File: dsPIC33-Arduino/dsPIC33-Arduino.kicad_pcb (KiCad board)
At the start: 2 copper layers, 68.6 x 53.3 mm, 58 parts, among them CON1 BARREL_JACK, P1 Power, P10 PIN20, P11 PIN5, P12 PWR_IN, P13 PIN2, P14 Power Select, P15 I2C, P16 PIN19, P17 UART/CAN, P2 Analog, P3 Digital, P4 Digital, P5 CONN_1, P6 CONN_1, P7 CONN_1, P8 CONN_1, P9 USB_B, SW1 SW_PUSH, U1 FT230XS, U2 LM1117 3V3, U3 dsPIC33EVxxxGM102-I/SP, U4 74LVC1G32, U5 LM1117 5V, Y1 Crystal

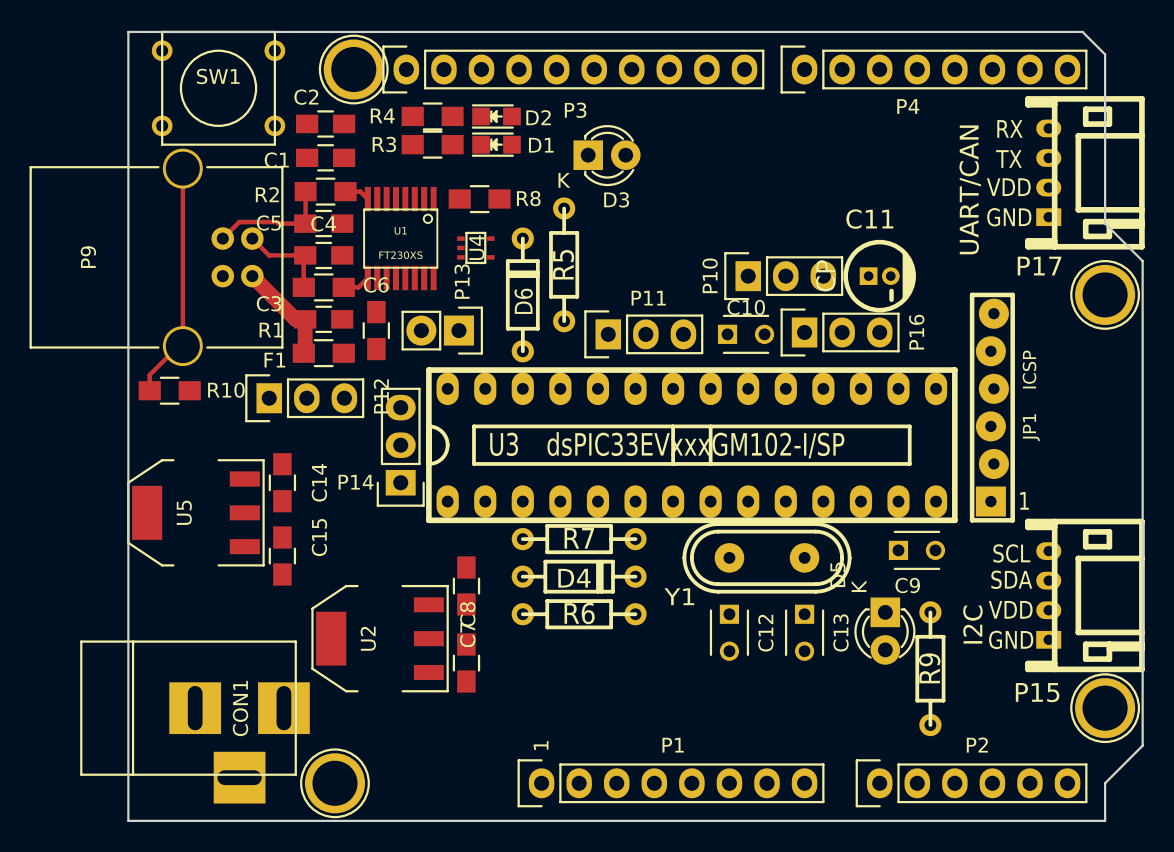
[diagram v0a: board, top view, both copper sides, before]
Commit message: wip
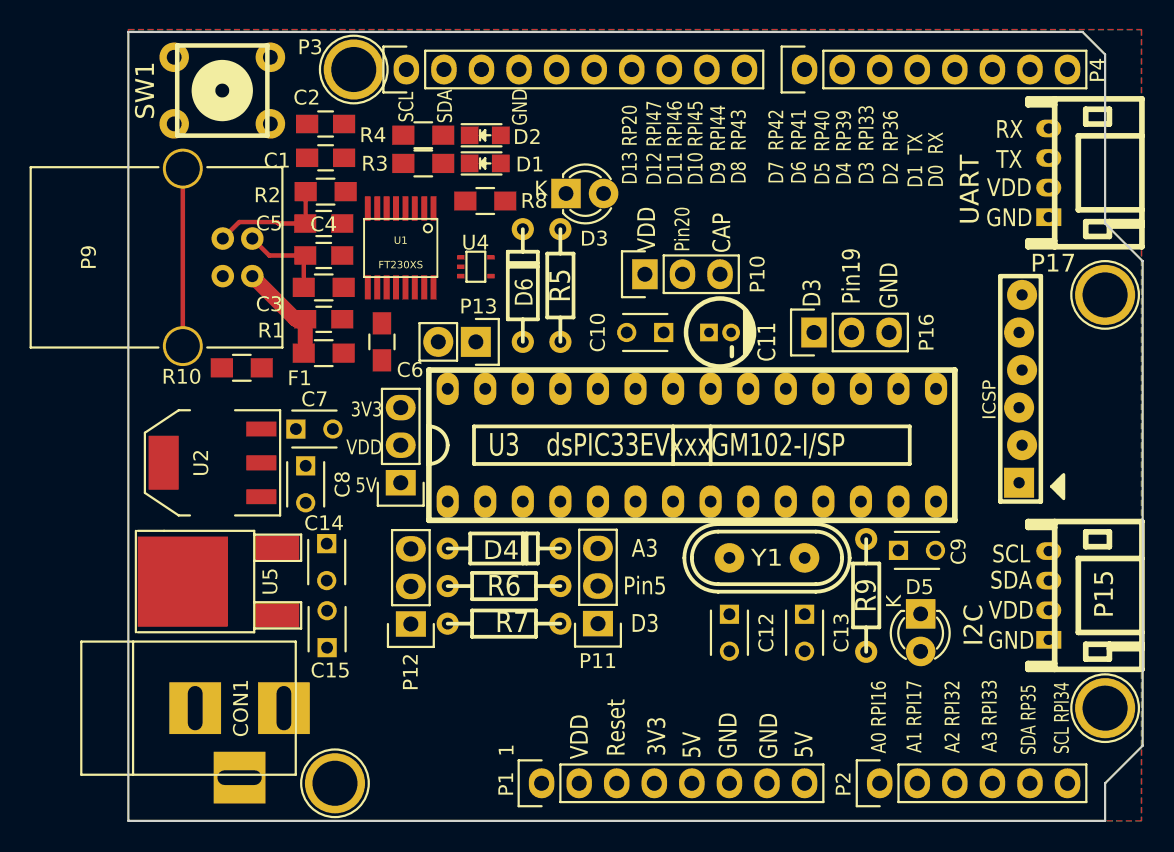
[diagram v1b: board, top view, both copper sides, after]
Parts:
- C14, C15, C7, C8: footprint Capacitors_SMD:C_0805_HandSoldering -> Capacitors_ThroughHole:C_Disc_D3_P2.5
- P17: value UART/CAN -> UART
- SW1: footprint Buttons_Switches_ThroughHole:SW_PUSH_SMALL -> w_switch:PCB_PUSH
- U5: value LM1117 5V -> 7805; footprint TO_SOT_Packages_SMD:SOT-223 -> 78xx:TO-252-2Lead
- moved P11 19.6 mm to (142.7, 113.0), turned to 180 degrees
- moved P12 18.0 mm to (130.1, 113.1), turned to 180 degrees
- moved C8 17.2 mm to (123.0, 102.4)
- moved U2 16.4 mm to (116.7, 102.2)
- moved C7 15.7 mm to (122.3, 99.9), turned to 0 degrees
- moved C14 11.6 mm to (124.4, 114.7), turned to 90 degrees
- moved C11 11.4 mm to (151.0, 93.3)
- moved R7 7.65 mm to (136.4, 113.0)
- moved U5 7.17 mm to (121.0, 110.2)
- moved P10 6.99 mm to (145.9, 89.4)
- moved R9 6.59 mm to (160.9, 111.1)
- moved D4 5.43 mm to (136.4, 108.0)
- moved R6 5.43 mm to (136.4, 110.5)
- moved R10 5.12 mm to (118.7, 95.7)
- moved C10 4.32 mm to (147.2, 93.3), turned to 180 degrees
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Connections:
- C14 pad 1: Net-(C14-Pad1) -> /VI
- CON1 pad 1: Net-(C14-Pad1) -> /VI
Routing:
- net Net-(P9-Pad5): track 16.1 -> 12.3 mm
- net Net-(R1-Pad1): track 1.90 -> 0.00 mm
- net Net-(R2-Pad1): track 1.72 -> 0.00 mm
- added copper zone on B.Cu, net GND
- added copper zone on F.Cu, net GND
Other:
- net class PWR2 added: clearance 0.2, trace_width 0.508, via_dia 0.6, via_drill 0.4
- board text added: "3V3"
- board text added: "5V"
- board text added: "A0 RPI16"
- board text added: "A1 RPI17"
- board text added: "A2 RPI32"
- board text added: "A3"
- board text added: "A3 RPI33"
- board text added: "CAP"
- board text added: "D0 RX"
- board text added: "D1 TX"
- board text added: "D10 RPI45"
- board text added: "D11 RPI46"
- board text added: "D12 RPI47"
- board text added: "D13 RP20"
- board text added: "D2 RP36"
- board text added: "D3"
- board text added: "D3 RPI33"
- board text added: "D4 RP39"
- board text added: "D5 RP40"
- board text added: "D6 RP41"
- board text added: "D7 RP42"
- board text added: "D8 RP43"
- board text added: "D9 RPI44"
- board text added: "Pin19"
- board text added: "Pin20"
- board text added: "Pin5"
- board text added: "Reset"
- board text added: "SCL RPI34"
- board text added: "SDA RP35"
